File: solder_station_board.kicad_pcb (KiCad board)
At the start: 2 copper layers, 55.9 x 44.2 mm, 43 parts, among them J1 PWR_5_V, J2 INPUT, J3 RT_WELLER, J4 INPUT, J5 VFD_DISPLAY, J6 PWR_15V, J8 SERIAL, P1 ISP, Q1 IRF9540, Q2 2N7002, U4 TLC272, U5 LT1007, U6 ATMEGA168-20AU

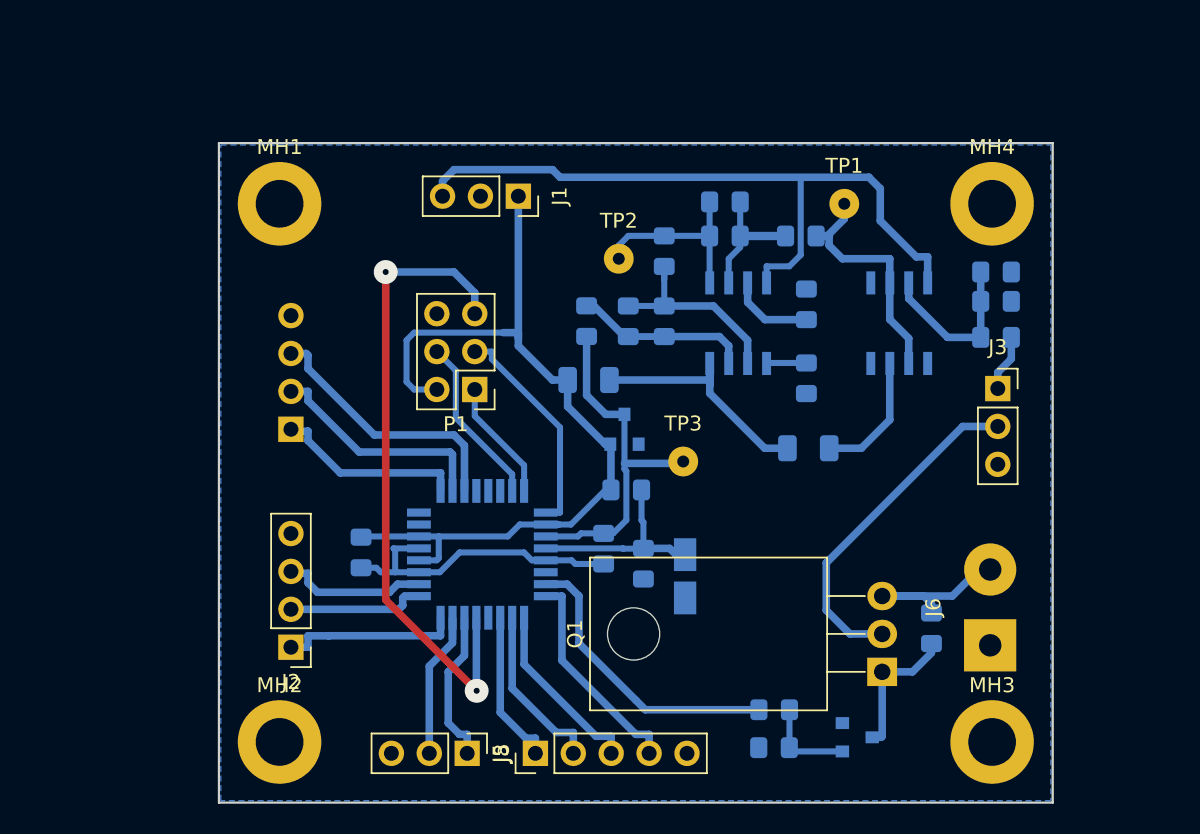
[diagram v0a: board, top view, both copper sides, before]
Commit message: jbc
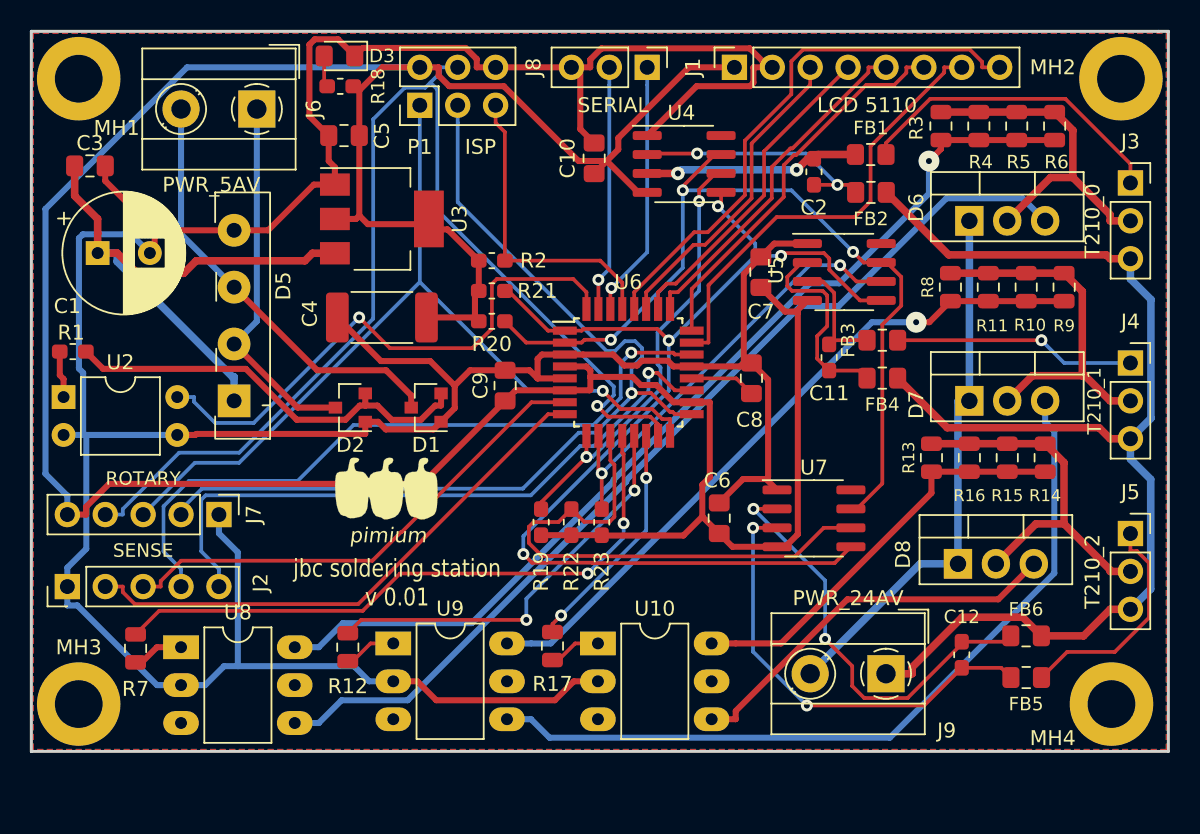
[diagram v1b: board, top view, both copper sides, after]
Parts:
- removed C13: 10n, Capacitor_SMD:C_0805_2012Metric_Pad1.15x1.40mm_HandSolder
- removed Q1: IRF9540, Package_TO_SOT_THT:TO-220-3_Horizontal_TabDown
- removed Q2: 2N7002, Package_TO_SOT_SMD:SOT-23
- removed TP1, TP2, TP3: tp, Connector_Wire:SolderWirePad_1x01_Drill0.8mm
- added C10: 100n, Capacitor_SMD:C_0805_2012Metric_Pad1.15x1.40mm_HandSolder, F.Cu at (68.0, 34.7)
- added C11: 10n, Capacitor_SMD:C_0603_1608Metric_Pad1.05x0.95mm_HandSolder, F.Cu at (83.8, 48.0)
- added C12: 10n, Capacitor_SMD:C_0603_1608Metric_Pad1.05x0.95mm_HandSolder, F.Cu at (92.7, 68.0)
- added C3: 100n, Capacitor_SMD:C_0805_2012Metric_Pad1.15x1.40mm_HandSolder, F.Cu at (34.2, 35.2)
- added C4: 10u, Capacitor_SMD:C_2512_6332Metric_Pad1.52x3.35mm_HandSolder, F.Cu at (53.8, 45.4)
- added C5: 100n, Capacitor_SMD:C_0805_2012Metric_Pad1.15x1.40mm_HandSolder, F.Cu at (51.3, 33.2)
- added C6: 100n, Capacitor_SMD:C_0805_2012Metric_Pad1.15x1.40mm_HandSolder, F.Cu at (76.4, 58.8)
- added D2: BAT54S, Package_TO_SOT_SMD:SOT-23, F.Cu at (51.7, 51.4)
- added D3: LED, LED_SMD:LED_0805_2012Metric_Pad1.15x1.40mm_HandSolder, F.Cu at (51.0, 27.8)
- added D5: GBU4A, custom:Diode_Bridge_Vishay_GBU_20P3.8mm, F.Cu at (43.9, 51.0)
- added D6: BT137, Package_TO_SOT_THT:TO-220-3_Vertical, F.Cu at (93.2, 38.9)
- added D7: BT137, Package_TO_SOT_THT:TO-220-3_Vertical, F.Cu at (93.2, 51.0)
- added FB1: ferrite, Inductor_SMD:L_0805_2012Metric_Pad1.15x1.40mm_HandSolder, F.Cu at (86.6, 34.4)
- added FB2: ferrite, Inductor_SMD:L_0805_2012Metric_Pad1.15x1.40mm_HandSolder, F.Cu at (86.6, 37.0)
- added FB3: ferrite, Inductor_SMD:L_0805_2012Metric_Pad1.15x1.40mm_HandSolder, F.Cu at (87.3, 46.9)
- added FB4: ferrite, Inductor_SMD:L_0805_2012Metric_Pad1.15x1.40mm_HandSolder, F.Cu at (87.3, 49.4)
- added FB5: ferrite, Inductor_SMD:L_0805_2012Metric_Pad1.15x1.40mm_HandSolder, F.Cu at (97.0, 69.5)
- added FB6: ferrite, Inductor_SMD:L_0805_2012Metric_Pad1.15x1.40mm_HandSolder, F.Cu at (97.0, 66.7)
- added G***: LOGO, custom_logo:pimium_paprika_7mm, F.Cu at (54.1, 58.1)
- added J7: ROTARY, Connector_PinHeader_2.54mm:PinHeader_1x05_P2.54mm_Vertical, F.Cu at (42.9, 58.6)
- added J9: PWR_24AV, TerminalBlock_MetzConnect:TerminalBlock_MetzConnect_Type101_RT01602HBWC_1x02_P5.08mm_Horizontal, F.Cu at (87.6, 69.2)
- added R17: 270, Resistor_SMD:R_0805_2012Metric, F.Cu at (65.2, 67.4)
- added R18: 330, Resistor_SMD:R_0603_1608Metric_Pad1.05x0.95mm_HandSolder, F.Cu at (51.0, 29.9)
- added R19: 1k, Resistor_SMD:R_0603_1608Metric_Pad1.05x0.95mm_HandSolder, F.Cu at (64.5, 59.1)
- added R20: 1k, Resistor_SMD:R_0603_1608Metric_Pad1.05x0.95mm_HandSolder, F.Cu at (61.2, 45.6)
- added R21: 1k, Resistor_SMD:R_0603_1608Metric_Pad1.05x0.95mm_HandSolder, F.Cu at (61.2, 43.6)
- added R22: 1k, Resistor_SMD:R_0603_1608Metric_Pad1.05x0.95mm_HandSolder, F.Cu at (66.5, 59.1)
- added R23: 1k, Resistor_SMD:R_0603_1608Metric_Pad1.05x0.95mm_HandSolder, F.Cu at (68.5, 59.1)
- added R3: 150, Resistor_SMD:R_0805_2012Metric, F.Cu at (91.3, 32.5)
- added U10: MOC3023M, Package_DIP:DIP-6_W7.62mm_LongPads, F.Cu at (68.3, 67.2)
- added U2: PC817, Package_DIP:DIP-4_W7.62mm, F.Cu at (32.5, 50.7)
- added U3: LT1117-3.3, Package_TO_SOT_SMD:SOT-223-3_TabPin2, F.Cu at (53.8, 38.8)
- added U7: MAX31855KASA, Package_SO:SOIC-8_3.9x4.9mm_P1.27mm, F.Cu at (82.8, 58.8)
- added U8: MOC3023M, Package_DIP:DIP-6_W7.62mm_LongPads, F.Cu at (40.3, 67.5)
- added U9: MOC3023M, Package_DIP:DIP-6_W7.62mm_LongPads, F.Cu at (54.6, 67.2)
- C1: value 10n -> 100u; footprint Capacitor_SMD:C_0805_2012Metric_Pad1.15x1.40mm_HandSolder -> Capacitor_THT:CP_Radial_D8.0mm_P3.50mm; moved to F.Cu
- C2: footprint Capacitor_SMD:C_0805_2012Metric_Pad1.15x1.40mm_HandSolder -> Capacitor_SMD:C_0603_1608Metric_Pad1.05x0.95mm_HandSolder; moved to F.Cu
- C7: value 10n -> 100n; moved to F.Cu
- C8, C9, D1, U6: moved to F.Cu
- D8: value 4V7 -> BT137; footprint Diode_SMD:D_MicroMELF_Hadsoldering -> Package_TO_SOT_THT:TO-220-3_Vertical; moved to F.Cu
- J1: value PWR_5_V -> LCD 5110; footprint Connector_PinSocket_2.54mm:PinSocket_1x03_P2.54mm_Vertical -> Connector_PinSocket_2.54mm:PinSocket_1x08_P2.54mm_Vertical
- J2: value INPUT -> SENSE; footprint Connector_PinHeader_2.54mm:PinHeader_1x04_P2.54mm_Vertical -> Connector_PinHeader_2.54mm:PinHeader_1x05_P2.54mm_Vertical
- J3: value RT_WELLER -> T210_0
- J4: value INPUT -> T210_1; footprint Connector_PinHeader_2.54mm:PinHeader_1x04_P2.54mm_Vertical -> Connector_PinSocket_2.54mm:PinSocket_1x03_P2.54mm_Vertical; moved to F.Cu
- J5: value VFD_DISPLAY -> T210_2; footprint Connector_PinHeader_2.54mm:PinHeader_1x05_P2.54mm_Vertical -> Connector_PinSocket_2.54mm:PinSocket_1x03_P2.54mm_Vertical
- J6: value PWR_15V -> PWR_5AV; footprint Connector_Wire:SolderWirePad_1x02_P5.08mm_Drill1.5mm -> TerminalBlock_MetzConnect:TerminalBlock_MetzConnect_Type101_RT01602HBWC_1x02_P5.08mm_Horizontal
- R1: value 0 -> 330; footprint Resistor_SMD:R_1206_3216Metric -> Resistor_SMD:R_0603_1608Metric_Pad1.05x0.95mm_HandSolder; moved to F.Cu
- R10, R11, R13, R16, R4, R9: value 1k -> 150; footprint Resistor_SMD:R_0805_2012Metric_Pad1.15x1.40mm_HandSolder -> Resistor_SMD:R_0805_2012Metric; moved to F.Cu
- R12: value 22k -> 270; footprint Resistor_SMD:R_0805_2012Metric_Pad1.15x1.40mm_HandSolder -> Resistor_SMD:R_0805_2012Metric; moved to F.Cu
- R14: value 33k -> 150; footprint Resistor_SMD:R_0805_2012Metric_Pad1.15x1.40mm_HandSolder -> Resistor_SMD:R_0805_2012Metric; moved to F.Cu
- R15: value 10K -> 150; footprint Resistor_SMD:R_0805_2012Metric_Pad1.15x1.40mm_HandSolder -> Resistor_SMD:R_0805_2012Metric; moved to F.Cu
- R2: value 0 -> 1k; footprint Resistor_SMD:R_1206_3216Metric -> Resistor_SMD:R_0603_1608Metric_Pad1.05x0.95mm_HandSolder; moved to F.Cu
- R5: value 5k6 -> 150; footprint Resistor_SMD:R_0805_2012Metric_Pad1.15x1.40mm_HandSolder -> Resistor_SMD:R_0805_2012Metric; moved to F.Cu
- R6: value 4k7 -> 150; footprint Resistor_SMD:R_0805_2012Metric_Pad1.15x1.40mm_HandSolder -> Resistor_SMD:R_0805_2012Metric; moved to F.Cu
- R7: value 100k -> 270; footprint Resistor_SMD:R_0805_2012Metric_Pad1.15x1.40mm_HandSolder -> Resistor_SMD:R_0805_2012Metric; moved to F.Cu
- R8: value 2k2 -> 150; footprint Resistor_SMD:R_0805_2012Metric_Pad1.15x1.40mm_HandSolder -> Resistor_SMD:R_0805_2012Metric; moved to F.Cu
- U4: value TLC272 -> MAX31855KASA; moved to F.Cu
- U5: value LT1007 -> MAX31855KASA; moved to F.Cu
- moved MH2 71.8 mm to (103.3, 29.4)
- moved R7 62.2 mm to (37.3, 67.5), turned to 270 degrees
- moved MH3 61.3 mm to (33.5, 71.3)
- moved J6 60.9 mm to (45.4, 31.4), turned to 180 degrees
- moved J4 56.4 mm to (104.0, 48.4)
- moved R1 49.7 mm to (33.1, 47.6)
- moved J8 47.5 mm to (71.6, 28.6)
- moved J5 42.5 mm to (104.0, 59.8), turned to 0 degrees
- moved C1 42.2 mm to (34.8, 41.0), turned to 0 degrees
- moved R12 37.4 mm to (51.5, 67.5), turned to 270 degrees
- moved R6 34.7 mm to (98.9, 32.5), turned to 90 degrees
- moved MH4 34.5 mm to (102.7, 71.3)
- moved R9 34.3 mm to (99.5, 43.3), turned to 90 degrees
- moved R8 33.0 mm to (91.9, 43.3), turned to 90 degrees
- moved R15 29.6 mm to (95.7, 54.8), turned to 90 degrees
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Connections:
- C1 pad 2: Net-(C1-Pad2) -> GND
- C7 pad 1: Net-(C7-Pad1) -> +3V3
- C9 pad 1: +5V -> +3V3
- D1 pad 2: +5V -> Net-(D1-Pad2)
- D1 pad 3: /TEMP -> Net-(D1-Pad3)
- D8 pad 1: Net-(C8-Pad1) -> Net-(D6-Pad1)
- D8 pad 2: GND -> /Sheet5FFC8D70/BLUE2
- J1 pad 1: +5V -> +3V3
- J1 pad 3: -5V -> /DIS_SCE
- J2 pad 1: /INP1 -> GND
- J2 pad 2: /INP2 -> /SENSE1
- J2 pad 3: /INP3 -> /SENSE0
- J2 pad 4: GND -> /ASENSE1
- J3 pad 1: Net-(J3-Pad1) -> /RED0
- J3 pad 2: Net-(J3-Pad2) -> /Sheet5FFC8D70/BLUE0
- J3 pad 3: GND -> GNDA
- J4 pad 1: /INP4 -> /RED1
- J4 pad 2: /INP5 -> /Sheet5FFC8D70/BLUE1
- J4 pad 3: /INP6 -> GNDA
- J5 pad 1: /VFD_DATA -> /RED2
- J5 pad 2: /VFD_RCLK -> /Sheet5FFC8D70/BLUE2
- J5 pad 3: /VFD_SRCLK -> GNDA
- J6 pad 1: GND -> Net-(D2-Pad3)
- J6 pad 2: +15V -> Net-(D1-Pad3)
- P1 pad 2: +5V -> +3V3
- R1 pad 1: +5V -> Net-(R1-Pad1)
- R1 pad 2: +5V -> Net-(D1-Pad2)
- R10 pad 2: Net-(C1-Pad1) -> /Sheet5FFC8D70/BLUE1
- R11 pad 1: +5V -> Net-(R10-Pad1)
- R11 pad 2: Net-(C8-Pad1) -> /Sheet5FFC8D70/BLUE1
- R12 pad 1: Net-(C1-Pad1) -> /SOLDER1
- R12 pad 2: Net-(C1-Pad2) -> Net-(R12-Pad2)
- R13 pad 1: Net-(C1-Pad2) -> Net-(R13-Pad1)
- R13 pad 2: Net-(C2-Pad1) -> /Sheet5FFC8D70/BLUE2
- R14 pad 1: Net-(C2-Pad1) -> Net-(R13-Pad1)
- R14 pad 2: Net-(C2-Pad2) -> /Sheet5FFC8D70/BLUE2
- R15 pad 1: Net-(C2-Pad2) -> Net-(R13-Pad1)
- R15 pad 2: /TEMP -> /Sheet5FFC8D70/BLUE2
- R16 pad 1: Net-(R16-Pad1) -> Net-(R13-Pad1)
- R16 pad 2: GND -> /Sheet5FFC8D70/BLUE2
- R2 pad 1: +5V -> /RST
- R2 pad 2: +5V -> +3V3
- R4 pad 1: Net-(R4-Pad1) -> Net-(R3-Pad1)
- R4 pad 2: GND -> /Sheet5FFC8D70/BLUE0
- R5 pad 1: Net-(C7-Pad1) -> Net-(R3-Pad1)
- R5 pad 2: Net-(J3-Pad1) -> /Sheet5FFC8D70/BLUE0
- R6 pad 1: +15V -> Net-(R3-Pad1)
- R6 pad 2: Net-(Q1-Pad1) -> /Sheet5FFC8D70/BLUE0
- R7 pad 1: GND -> /SOLDER0
- R7 pad 2: Net-(C7-Pad1) -> Net-(R7-Pad2)
- R8 pad 1: GND -> Net-(R10-Pad1)
- R8 pad 2: Net-(Q2-Pad1) -> /Sheet5FFC8D70/BLUE1
- R9 pad 1: /SOLDER -> Net-(R10-Pad1)
- R9 pad 2: Net-(Q2-Pad1) -> /Sheet5FFC8D70/BLUE1
- U4 pad 1: Net-(C1-Pad2) -> GND
- U4 pad 2: Net-(C1-Pad1) -> Net-(C2-Pad2)
- U4 pad 3: Net-(R4-Pad1) -> Net-(C2-Pad1)
- U4 pad 4: -5V -> +3V3
- U4 pad 5: Net-(R16-Pad1) -> /MAX_SCK
- U4 pad 6: Net-(C2-Pad1) -> /MAX_CS0
- U4 pad 7: Net-(C2-Pad2) -> /MAX_SO
- U4 pad 8: +5V -> (no net)
- U5 pad 1: (no net) -> GND
- U5 pad 2: Net-(R10-Pad1) -> Net-(C11-Pad2)
- U5 pad 3: Net-(C7-Pad1) -> Net-(C11-Pad1)
- U5 pad 4: -5V -> +3V3
- U5 pad 5: (no net) -> /MAX_SCK
- U5 pad 6: Net-(R10-Pad1) -> /MAX_CS1
- U5 pad 7: +5V -> /MAX_SO
- U6 pad 1: /INP2 -> /MAX_SCK
- U6 pad 10: /INP5 -> /MAX_CS1
- U6 pad 11: /INP6 -> /MAX_CS2
- U6 pad 12: (no net) -> /SOLDER0
- U6 pad 13: (no net) -> /SOLDER1
- U6 pad 14: (no net) -> /SOLDER2
- U6 pad 18: +5V -> +3V3
- U6 pad 19: /TEMP -> /ASENSE0
- U6 pad 2: /INP3 -> /MAX_SO
- U6 pad 22: (no net) -> /ASENSE1
- U6 pad 23: /SOLDER -> /DIS_CLK
- U6 pad 24: /VFD_SRCLR -> /DIS_DIN
- U6 pad 25: /VFD_SRCLK -> /DIS_D\C
- U6 pad 26: /VFD_RCLK -> /DIS_RST
- U6 pad 27: /VFD_DATA -> /DIS_SCE
- U6 pad 28: (no net) -> /DIS_LED
- U6 pad 32: /INP1 -> /TACK
- U6 pad 4: +5V -> +3V3
- U6 pad 6: +5V -> +3V3
- U6 pad 7: (no net) -> /SENSE0
- U6 pad 8: (no net) -> /SENSE1
- U6 pad 9: /INP4 -> /MAX_CS0
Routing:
- net GND: track 20.5 -> 249.7 mm
- net +3V3: track 0.00 -> 211.1 mm
- net +5V: track 85.1 -> 0.00 mm
- net GNDA: track 0.00 -> 80.7 mm
- net /MAX_SCK: track 0.00 -> 77.2 mm, vias 0 -> 4
- net Net-(R3-Pad1): track 0.00 -> 66.7 mm, vias 0 -> 1
- net /MOSI: track 11.4 -> 77.1 mm, vias 0 -> 1
- net Net-(D6-Pad3): track 0.00 -> 65.5 mm
- net /MAX_SO: track 0.00 -> 57.7 mm, vias 0 -> 3
- net Net-(D7-Pad3): track 0.00 -> 53.6 mm
- net /SCK: track 14.8 -> 65.3 mm, vias 0 -> 1
- net /MISO: track 8.17 -> 58.5 mm, vias 0 -> 1
- net -5V: track 48.1 -> 0.00 mm
- net /ASENSE1: track 0.00 -> 46.9 mm, vias 0 -> 1
- net /ASENSE0: track 0.00 -> 43.9 mm, vias 0 -> 1
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- added copper zone on F.Cu, net GND
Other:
- board size 55.9 x 44.2 mm -> 76.2 x 48.3 mm
- net class POWER added: clearance 0.2532, trace_width 0.508, via_dia 0.9016, via_drill 0.4
- net class Signal: clearance 0.2 -> 0.21; trace_width 0.25 -> 0.4064
- board text added: "jbc soldering station v 0.01"
